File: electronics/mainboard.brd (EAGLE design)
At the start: 160 x 160 mm, 18 parts, among them T1 NPN_BC817,215

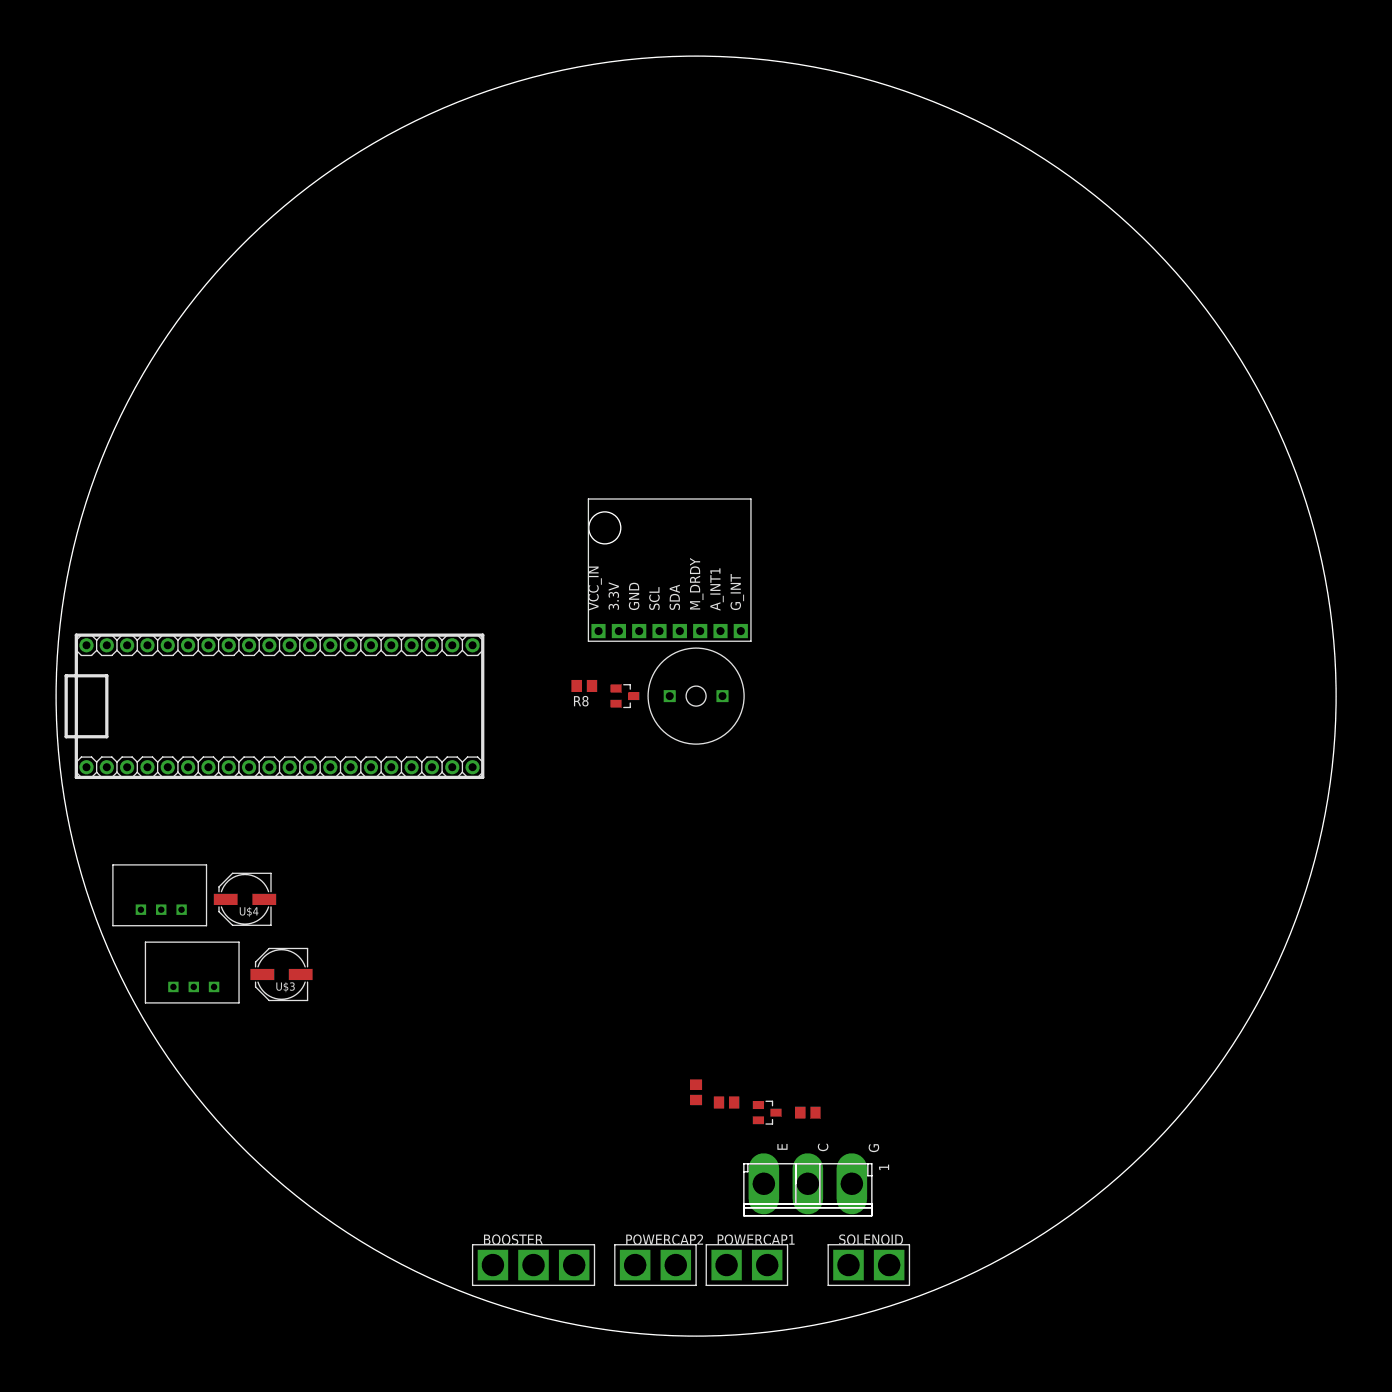
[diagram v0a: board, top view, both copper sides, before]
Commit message: Board wip
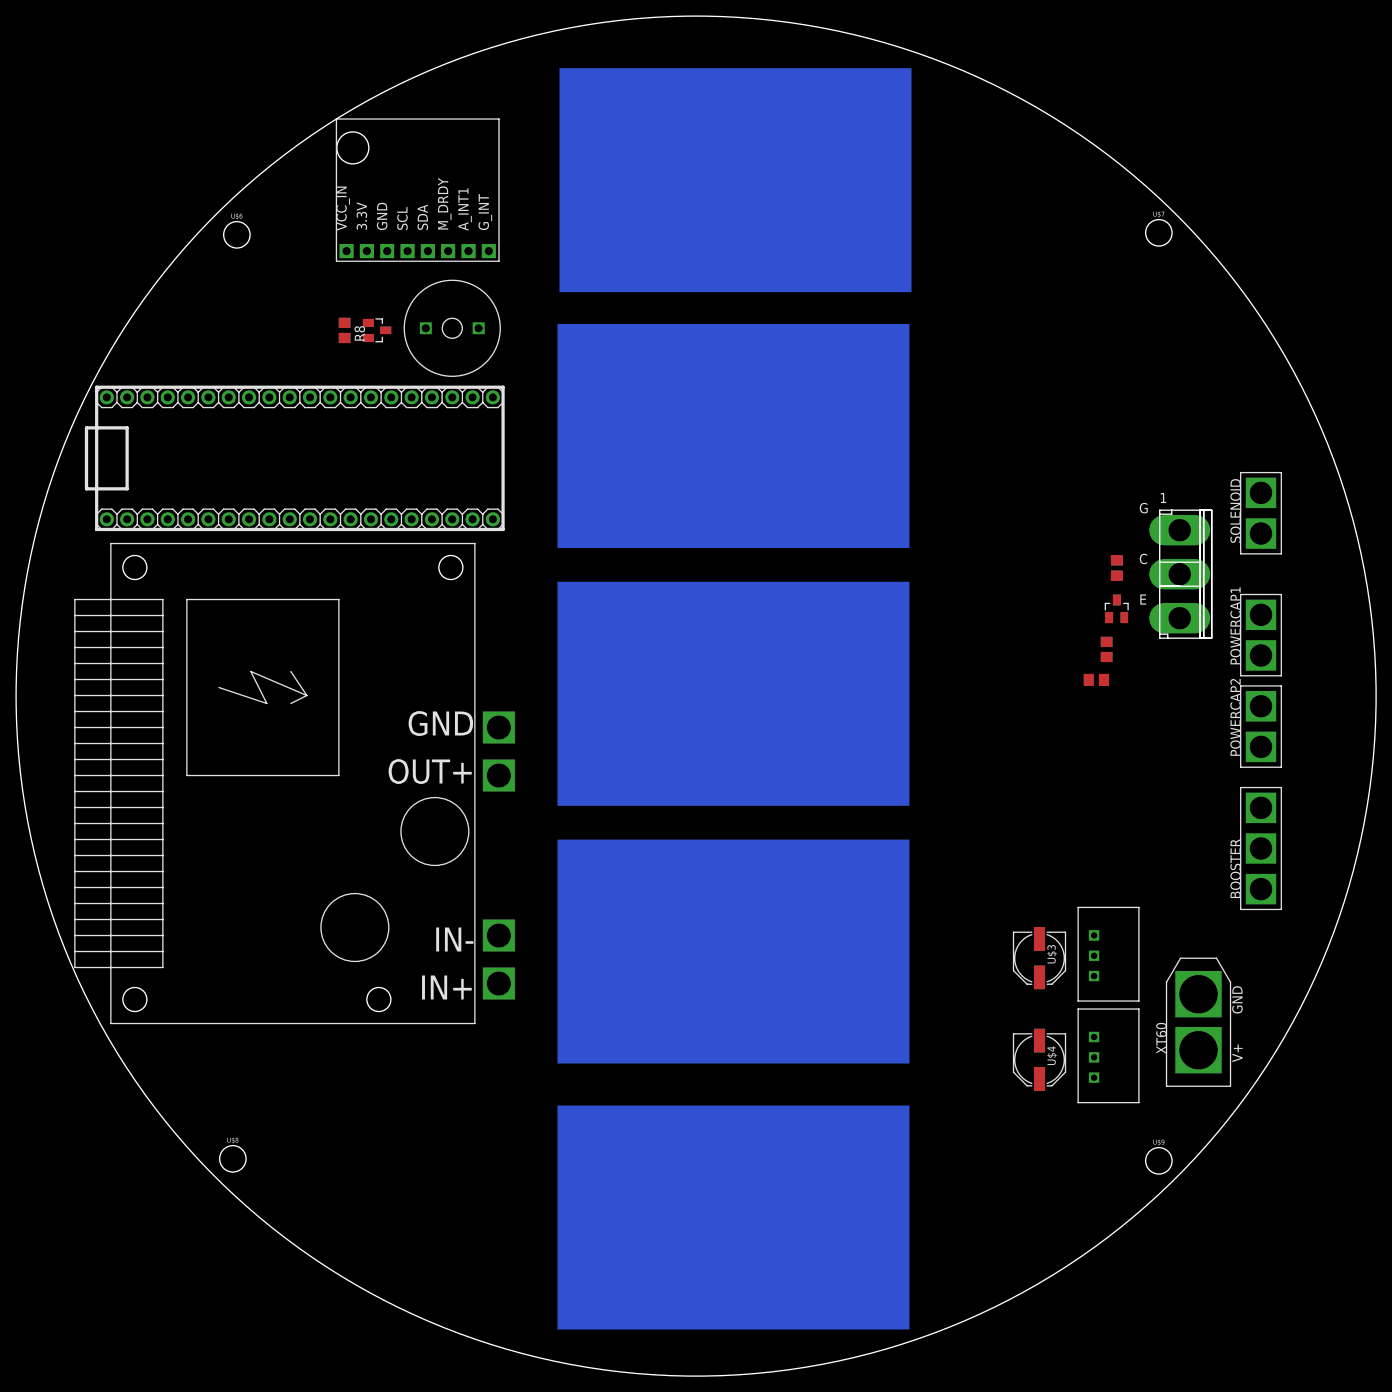
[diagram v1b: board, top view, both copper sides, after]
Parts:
- added U$5: BOOSTER, rhoban:BOOSTER_390V
- added U$6, U$7, U$8, U$9: (no value), SparkFun-Hardware:STAND-OFF
- added XT60: CONNEC_ALIM, rhoban:XT60
- moved REG5V 121.1 mm to (47.8, -39.1), turned to 270 degrees
- moved REG3.3V 117.2 mm to (47.8, -26.4), turned to 270 degrees
- moved BOOSTER 105.8 mm to (70.6, -21.6), turned to 90 degrees
- moved SOLENOID 105.0 mm to (70.6, 20.3), turned to 90 degrees
- moved POWERCAP2 101.6 mm to (70.6, -6.35), turned to 90 degrees
- moved POWERCAP1 101.3 mm to (70.6, 5.08), turned to 90 degrees
- moved U$4 101.3 mm to (42.9, -45.5), turned to 270 degrees
- moved U$3 94.8 mm to (42.9, -32.8), turned to 270 degrees
- moved U$1 89.3 mm to (60.5, 15.2), turned to 0 degrees
- moved R3 78.3 mm to (52.6, 16.0), turned to 90 degrees
- moved T1 76.7 mm to (52.6, 10.9), turned to 0 degrees
- moved R1 73.9 mm to (51.3, 5.84), turned to 90 degrees
- moved R2 71.9 mm to (50.0, 2.03), turned to 180 degrees
- moved U$2 57.0 mm to (-25.9, 55.6)
- moved U$12 55.2 mm to (-39.9, 45.7)
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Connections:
- net GND: now also U$5.IN-, U$5.OUT-, XT60.GND
- net VBOOST: now also U$5.OUT+
- net VIN: now also U$5.VIN, XT60.V+
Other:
- board size 160 x 160 mm -> 170 x 170 mm
